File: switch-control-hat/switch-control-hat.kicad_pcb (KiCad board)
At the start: 2 copper layers, 85 x 56 mm, 40 parts, among them J1 Frontend Connector, J2 Power Connector, J3 Conn_01x02, P1 RPi-Header, U1 TLP3543, U2 TLP3543, U3 TLP3543, U4 TLP3543, U5 TLP3543, U6 TLP3543, U7 TLP3543, U8 TLP3543, U9 DS3231M

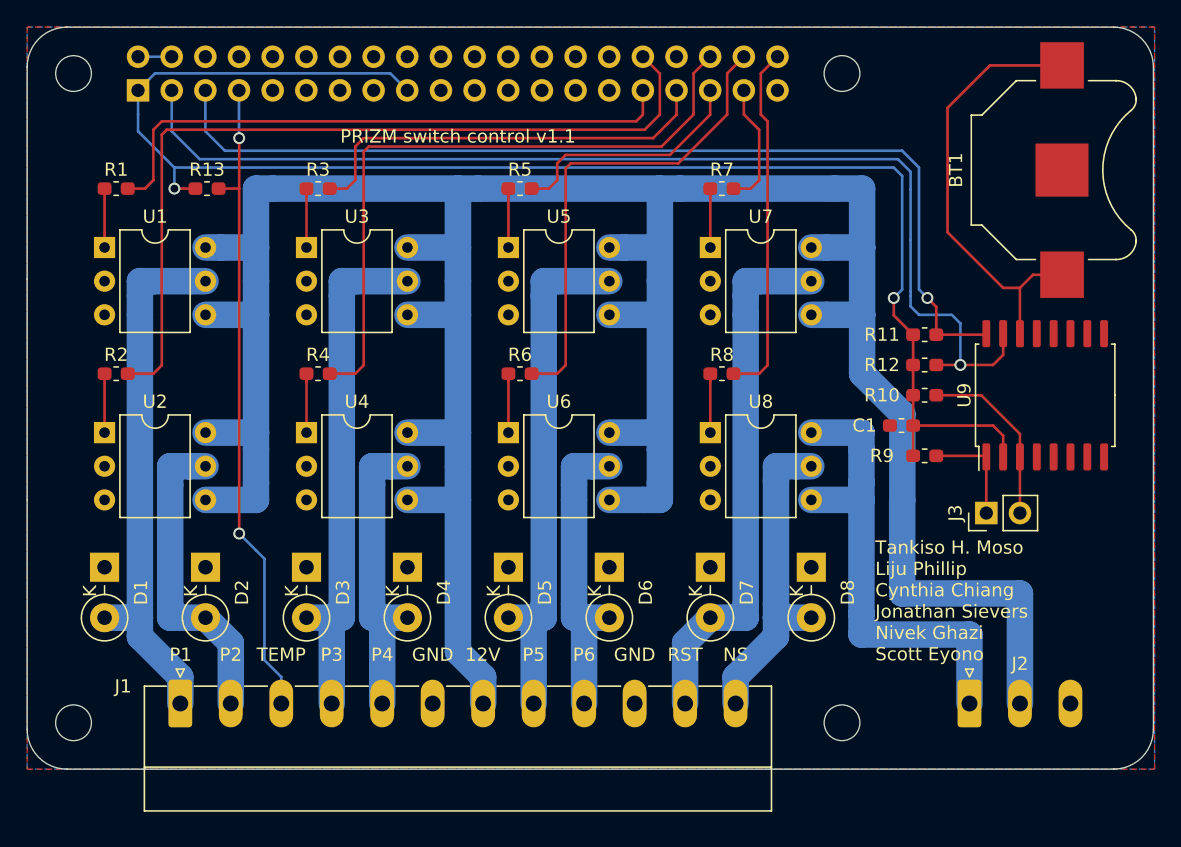
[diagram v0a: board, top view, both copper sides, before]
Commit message: final version
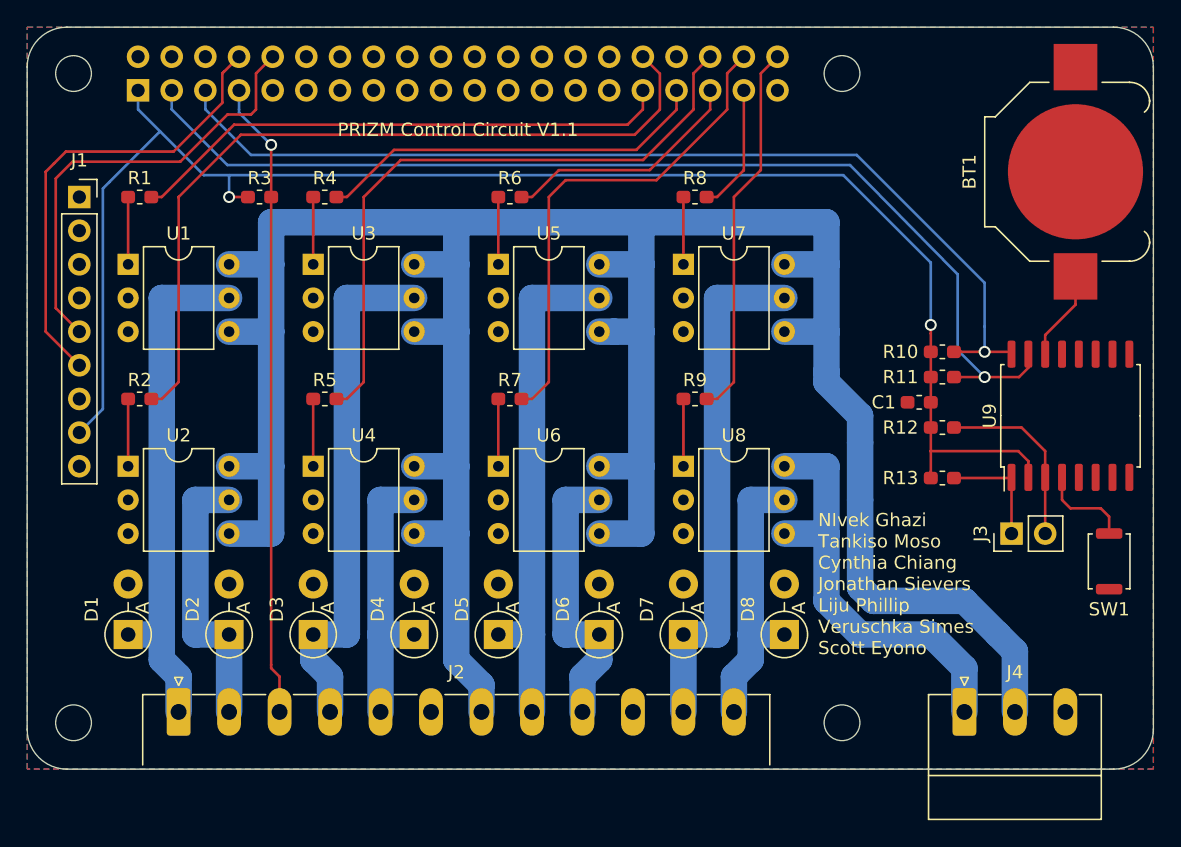
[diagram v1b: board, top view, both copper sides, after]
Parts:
- added J4: Power Connector, Connector_Phoenix_MC:PhoenixContact_MC_1,5_3-G-3.81_1x03_P3.81mm_Horizontal, F.Cu at (270.7, 145.7)
- added SW1: SW_Push, Button_Switch_SMD:SW_Push_SPST_NO_Alps_SKRK, F.Cu at (281.7, 134.3)
- D1, D2, D3, D4, D5, D6, D7, D8: footprint Diode_THT:D_DO-41_SOD81_P3.81mm_Vertical_KathodeUp -> Diode_THT:D_DO-41_SOD81_P3.81mm_Vertical_AnodeUp
- J1: value Frontend Connector -> Conn_01x09; footprint Connector_Phoenix_MC:PhoenixContact_MC_1,5_12-G-3.81_1x12_P3.81mm_Horizontal -> Connector_PinSocket_2.54mm:PinSocket_1x09_P2.54mm_Vertical
- J2: value Power Connector -> Frontend Connector; footprint Connector_Phoenix_MC:PhoenixContact_MC_1,5_3-G-3.81_1x03_P3.81mm_Horizontal -> Connector_Phoenix_MC:PhoenixContact_MC_1,5_12-G-3.81_1x12_P3.81mm_Horizontal
- R3: value 200 -> 4K7
- R9: value 4K7 -> 200
- moved J2 59.7 mm to (211.4, 145.7)
- moved R13 59.6 mm to (269.1, 128.0), turned to 180 degrees
- moved J1 39.0 mm to (203.9, 106.8)
- moved R7 22.5 mm to (236.4, 122.1)
- moved R5 21.7 mm to (222.5, 122.1)
- moved R9 17.9 mm to (250.4, 122.1), turned to 0 degrees
- moved R8 13.5 mm to (250.4, 106.8)
- moved R6 13.4 mm to (236.4, 106.8)
- moved R4 13.3 mm to (222.5, 106.8)
- moved D8 5.47 mm to (257.1, 139.8), turned to 90 degrees
- moved D7 5.47 mm to (249.5, 139.8), turned to 90 degrees
- moved D2 5.38 mm to (215.2, 139.8), turned to 90 degrees
- moved D1 5.38 mm to (207.6, 139.8), turned to 90 degrees
- moved D5 5.14 mm to (235.6, 139.8), turned to 90 degrees
- moved D6 5.14 mm to (243.2, 139.8), turned to 90 degrees
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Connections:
- D1 pad 1: GND -> /POS1
- D1 pad 2: /POS1 -> GND
- D2 pad 1: GND -> /POS2
- D2 pad 2: /POS2 -> GND
- D3 pad 1: GND -> /POS3
- D3 pad 2: /POS3 -> GND
- D4 pad 1: GND -> /POS4
- D4 pad 2: /POS4 -> GND
- D5 pad 1: GND -> /POS5
- D5 pad 2: /POS5 -> GND
- D6 pad 1: GND -> /POS6
- D6 pad 2: /POS6 -> GND
- D7 pad 1: GND -> /RESET
- D7 pad 2: /RESET -> GND
- D8 pad 1: GND -> /NOISE-DIODE
- D8 pad 2: /NOISE-DIODE -> GND
- J1 pad 1: /POS1 -> (no net)
- J1 pad 2: /POS2 -> (no net)
- J1 pad 3: /ONE-WIRE -> (no net)
- J1 pad 4: /POS3 -> (no net)
- J1 pad 5: /POS4 -> /GPIO15(RXD0)
- J1 pad 6: GND -> /GPIO14(TXD0)
- J1 pad 7: +12V -> GND
- J1 pad 8: /POS5 -> +3V3
- J1 pad 9: /POS6 -> (no net)
- J2 pad 1: +15V -> /POS1
- J2 pad 2: +12V -> /POS2
- J2 pad 3: (no net) -> /ONE-WIRE
- P1 pad 10: (no net) -> /GPIO15(RXD0)
- P1 pad 17: +3V3 -> (no net)
- P1 pad 2: +5V -> (no net)
- P1 pad 4: +5V -> (no net)
- P1 pad 8: (no net) -> /GPIO14(TXD0)
- R10 pad 1: Net-(J3-Pad2) -> +3V3
- R10 pad 2: +3V3 -> /GPIO3(SCL1)
- R11 pad 2: /GPIO3(SCL1) -> /GPIO2(SDA1)
- R12 pad 1: +3V3 -> Net-(J3-Pad2)
- R12 pad 2: /GPIO2(SDA1) -> +3V3
- R13 pad 1: +3V3 -> Net-(J3-Pad1)
- R13 pad 2: /ONE-WIRE -> +3V3
- R3 pad 1: Net-(R3-Pad1) -> +3V3
- R3 pad 2: /GPIO13(PWM1) -> /ONE-WIRE
- R4 pad 2: /GPIO16 -> /GPIO13(PWM1)
- R5 pad 2: /GPIO19(SPI1_MISO) -> /GPIO16
- R6 pad 2: /GPIO20(SPI1_MOSI) -> /GPIO19(SPI1_MISO)
- R7 pad 2: /GPIO26 -> /GPIO20(SPI1_MOSI)
- R8 pad 2: /GPIO21(SPI1_SCK) -> /GPIO26
- R9 pad 1: Net-(J3-Pad1) -> Net-(R9-Pad1)
- R9 pad 2: +3V3 -> /GPIO21(SPI1_SCK)
- U3 pad 1: Net-(R3-Pad1) -> Net-(R4-Pad1)
- U4 pad 1: Net-(R4-Pad1) -> Net-(R5-Pad1)
- U5 pad 1: Net-(R5-Pad1) -> Net-(R6-Pad1)
- U6 pad 1: Net-(R6-Pad1) -> Net-(R7-Pad1)
- U7 pad 1: Net-(R7-Pad1) -> Net-(R8-Pad1)
- U8 pad 1: Net-(R8-Pad1) -> Net-(R9-Pad1)
- U9 pad 4: (no net) -> Net-(SW1-Pad1)
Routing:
- net /GPIO14(TXD0): track 0.00 -> 35.1 mm
- net /GPIO15(RXD0): track 0.00 -> 34.1 mm
- net Net-(BT1-Pad1): track 33.6 -> 6.81 mm
- net +12V: track 234.7 -> 218.0 mm
- net Net-(SW1-Pad1): track 0.00 -> 7.05 mm
- net Net-(R9-Pad1): track 0.00 -> 5.08 mm
- net Net-(R3-Pad1): track 4.44 -> 0.00 mm
- net /GPIO6: track 45.3 -> 41.3 mm
- net /GPIO12(PWM0): track 63.4 -> 60.1 mm
- net /GPIO2(SDA1): track 84.6 -> 81.5 mm
- net /POS2: track 24.0 -> 21.1 mm
- net /NOISE-DIODE: track 24.5 -> 21.6 mm
- net +5V: track 2.54 -> 0.00 mm
- net +15V: track 36.2 -> 33.6 mm
- net /POS4: track 23.3 -> 21.1 mm
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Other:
- outline, holes or cut-outs redrawn
- board text added: "NIvek Ghazi Tankiso Moso Cynthia Chiang Jonathan Sievers Liju Phillip Veruschka Simes Scott Eyono"
- board text added: "PRIZM Control Circuit V1.1"
- board text removed: "12V"
- board text removed: "GND"
- board text removed: "NS"
- board text removed: "P1"
- board text removed: "P2"
- board text removed: "P3"
- board text removed: "P4"
- board text removed: "P5"
- board text removed: "P6"
- board text removed: "PRIZM switch control v1.1"
- board text removed: "RST"
- board text removed: "TEMP"
- board text removed: "Tankiso H. Moso Liju Phillip Cynthia Chiang Jonathan Sievers Nivek Ghazi Scott Eyono"
